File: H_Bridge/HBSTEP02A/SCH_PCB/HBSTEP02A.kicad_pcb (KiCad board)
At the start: 2 copper layers, 61 x 61 mm, 78 parts, among them J1 VIO 3.3-5V, J10 SDO/NAO/CFG0, J11 ENCN/DCO, J12 ENCB/DCEN/CFG4, J13 ENCA/DCIN/CFG5, J14 SWP/DIAG1, J15 SWN/DIAG0, J16 CONN1_1, J17 CONN1_1, J18 POWER SELECT, J19 SDMODE, J2 REFL/STEP, J20 DRV_ENN_CFG6, J21 SWSEL, J22 SPIMODE, J23 AIN, J24 CONN1_1, J25 CONN1_1, J3 REFR/DIR, J4 CLK, J5 CONN1_1, J6 CONN1_1, J7 CSN/CFG3, J8 SCK/CFG2, J9 SID/NAI/CFG1, M1 HOLE, M2 HOLE, M3 HOLE, M4 HOLE, U1 TMC5130A

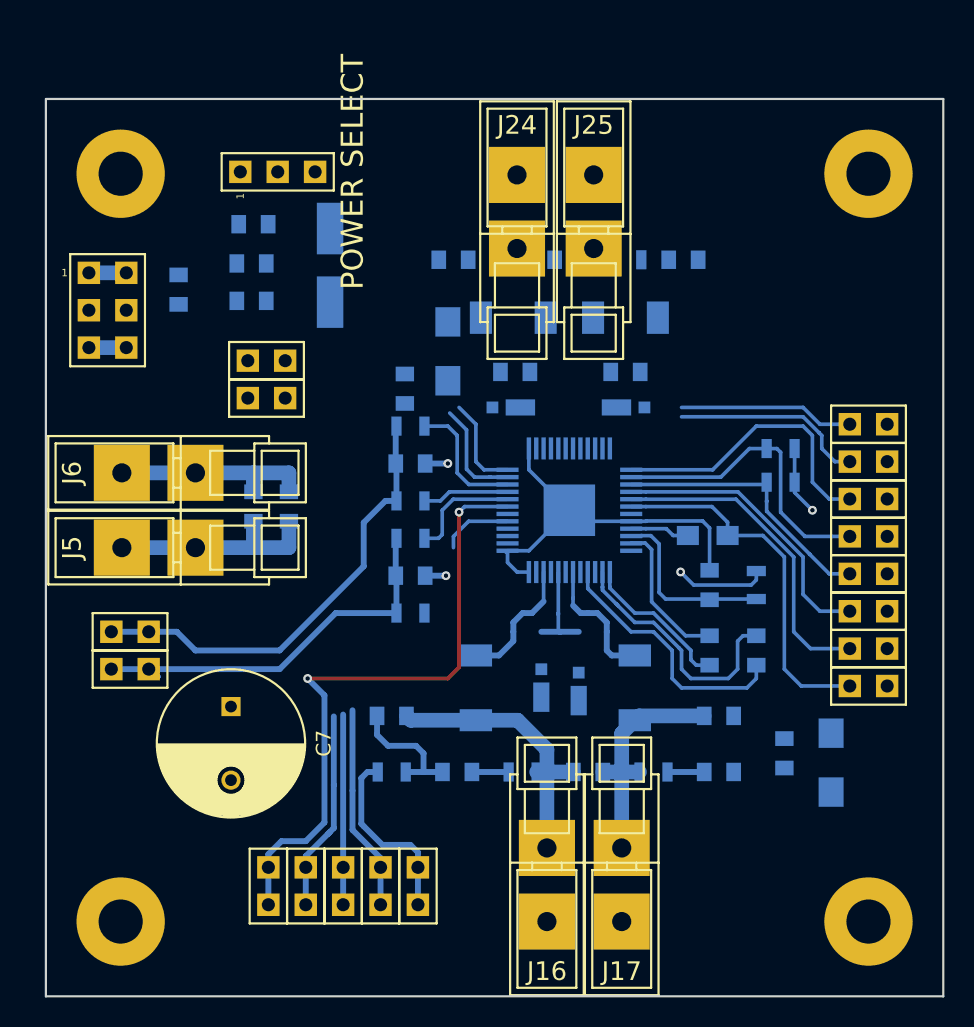
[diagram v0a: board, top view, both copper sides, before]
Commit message: layout update
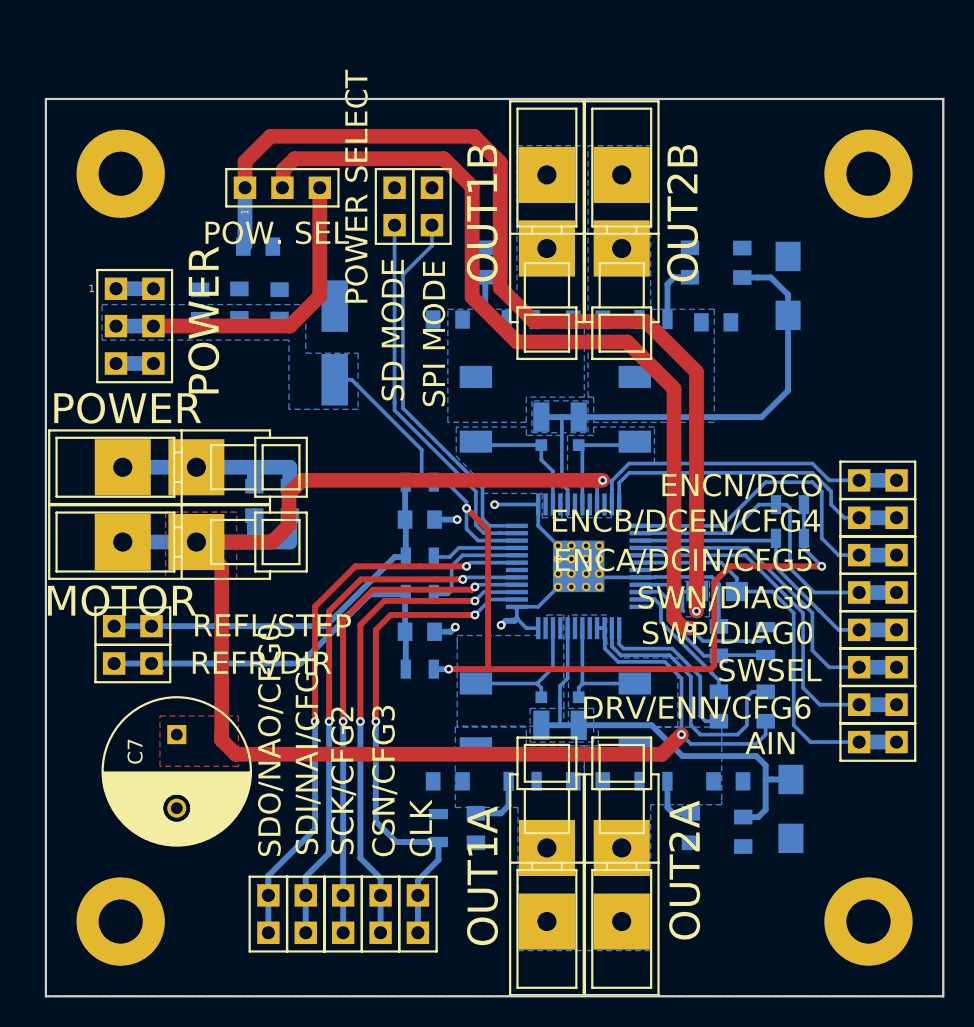
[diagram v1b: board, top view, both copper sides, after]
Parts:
- U1: footprint Housings_QFP:TQFP-48-1EP_7x7mm_Pitch0.5mm -> be3D TSSOP:TQFP-48-1EP_7x7mm_Pitch0.5mm_TRINAMIC
- moved C14 24.5 mm to (143.8, 100.0)
- moved R10 23.5 mm to (146.9, 101.6)
- moved J19 15.7 mm to (120.2, 96.2), turned to 0 degrees
- moved J22 15.4 mm to (122.7, 96.2), turned to 0 degrees
- moved C18 7.02 mm to (142.0, 104.1)
- moved L3 6.72 mm to (125.7, 110.0), turned to 270 degrees
- moved L4 6.26 mm to (136.5, 110.0), turned to 270 degrees
- moved C13 6.02 mm to (143.9, 138.7)
- moved C15 5.85 mm to (123.8, 135.3)
- moved C17 5.79 mm to (123.8, 103.9)
- moved D1 5.28 mm to (116.1, 105.5)
- moved R1 4.96 mm to (123.2, 138.4), turned to 90 degrees
- moved D4 4.60 mm to (132.7, 112.0), turned to 270 degrees
- moved C16 4.49 mm to (142.9, 135.3)
- moved R15 4.44 mm to (137.8, 103.9)
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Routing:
- net VSS: track 32.6 -> 112.6 mm, vias 0 -> 2
- net VCOM: track 13.5 -> 90.0 mm, vias 1 -> 3
- net +5V: track 4.04 -> 70.5 mm, vias 0 -> 1
- net VCC: track 6.26 -> 62.2 mm
- net Net-(C14-Pad1): track 0.00 -> 33.7 mm
- net Net-(C13-Pad1): track 6.83 -> 29.8 mm
- net Net-(J4-Pad1): track 12.6 -> 35.3 mm, vias 0 -> 2
- net Net-(J8-Pad1): track 12.9 -> 34.1 mm, vias 0 -> 2
- net Net-(J7-Pad1): track 14.0 -> 33.7 mm, vias 0 -> 2
- net Net-(C15-Pad2): track 19.7 -> 0.00 mm
- net Net-(J22-Pad2): track 6.54 -> 25.5 mm
- net Net-(J19-Pad2): track 7.38 -> 26.0 mm
- net Net-(J9-Pad1): track 18.6 -> 37.0 mm, vias 0 -> 2
- net Net-(C16-Pad1): track 16.4 -> 0.00 mm
- net Net-(J11-Pad1): track 11.9 -> 21.9 mm
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- added copper zone on B.Cu, net +5V
- added copper zone on B.Cu, net GNDA
- added copper zone on F.Cu, net GNDA
- added copper zone on B.Cu, net Net-(C13-Pad1)
- added copper zone on B.Cu, net Net-(C14-Pad1)
- added copper zone on B.Cu, net Net-(C15-Pad2)
- added copper zone on B.Cu, net Net-(C16-Pad1)
- added copper zone on B.Cu, net Net-(C17-Pad2)
- added copper zone on B.Cu, net Net-(C18-Pad2)
- added copper zone on B.Cu, net Net-(D2-Pad1)
- added copper zone on B.Cu, net Net-(D3-Pad1)
- added copper zone on B.Cu, net Net-(D4-Pad1)
- added copper zone on B.Cu, net Net-(D5-Pad1)
- added copper zone on B.Cu, net VCOM
- added copper zone on F.Cu, net VSS
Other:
- board text added: "AIN"
- board text added: "CLK"
- board text added: "CSN/CFG3"
- board text added: "DRV/ENN/CFG6"
- board text added: "ENCA/DCIN/CFG5"
- board text added: "ENCB/DCEN/CFG4"
- board text added: "ENCN/DCO"
- board text added: "MOTOR"
- board text added: "OUT1A"
- board text added: "OUT1B"
- board text added: "OUT2A"
- board text added: "OUT2B"
- board text added: "POW. SEL"
- board text added: "POWER"
- board text added: "REFL/STEP"
- board text added: "REFR/DIR"
- board text added: "SCK/CFG2"
- board text added: "SD MODE"
- board text added: "SDI/NAI/CFG1"
- board text added: "SDO/NAO/CFG0"
- board text added: "SPI MODE"
- board text added: "SWN/DIAG0"
- board text added: "SWP/DIAG0"
- board text added: "SWSEL"
